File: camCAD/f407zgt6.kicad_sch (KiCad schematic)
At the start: 2 parts, among them J2 SWD Header, U3 STM32F407ZGTx

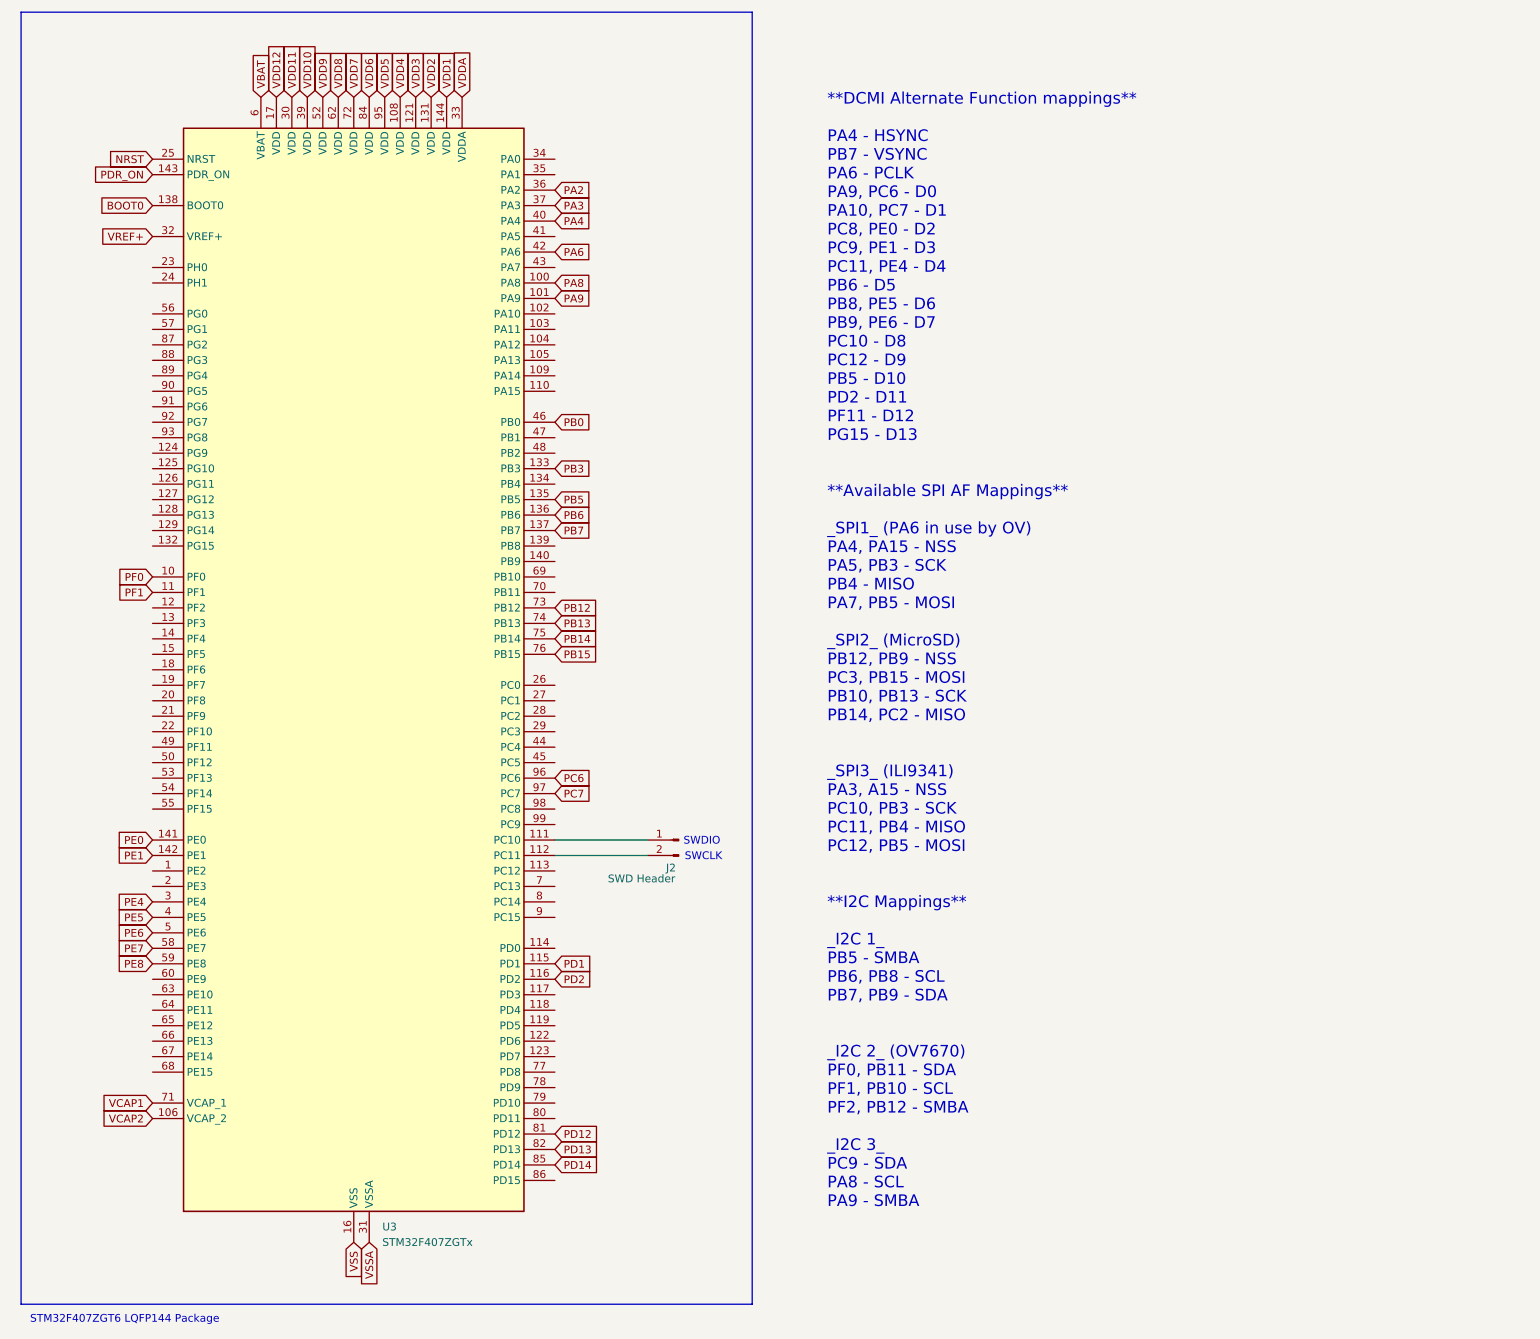
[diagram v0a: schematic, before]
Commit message: miscellaneous changes
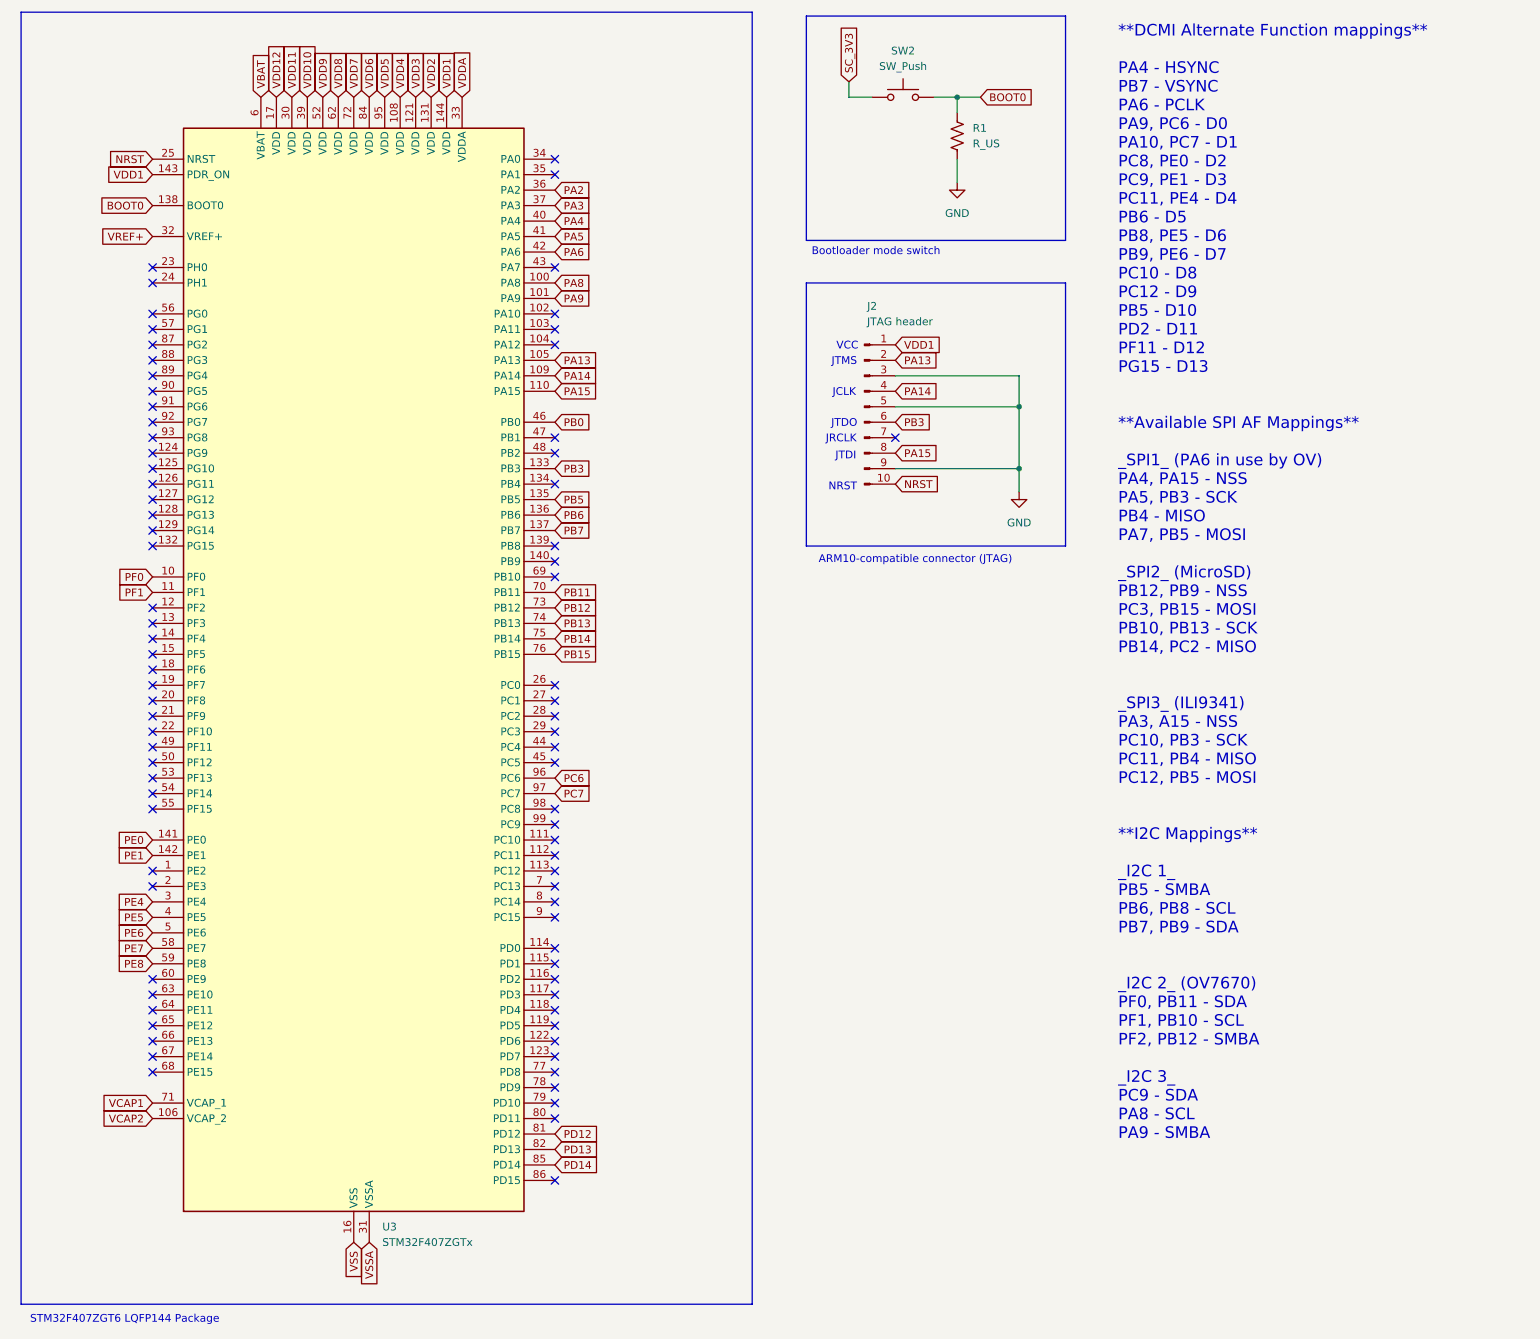
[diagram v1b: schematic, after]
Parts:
- removed J2: SWD Header, symbol Connector:Conn_01x02_Pin
- added J2: JTAG header, symbol Connector:Conn_01x10_Pin
- added R1: R_US, symbol Device:R_US
- added SW2: SW_Push, symbol Switch:SW_Push
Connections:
- net PDR_ON is gone; now on net VDD1: U3.143 (PDR_ON)
- net BOOT0: now also R1.1, SW2.2
- net NRST: now also J2.10 (Pin_10)
- net PB3: now also J2.6 (Pin_6)
- net VDD1: now also J2.1 (Pin_1)
- net PA13: now reaches U3.105 (PA13)
- net PA13: now also J2.2 (Pin_2)
- net PA14: now reaches U3.109 (PA14)
- net PA14: now also J2.4 (Pin_4)
- net PA15: now reaches U3.110 (PA15)
- net PA15: now also J2.8 (Pin_8)
- net PA5: now reaches U3.41 (PA5)
- net PB11: now reaches U3.70 (PB11)
- net PD1: no longer names the net of U3.115 (PD1)
- net PD2: no longer names the net of U3.116 (PD2)
- new net GND: J2.3 (Pin_3), J2.5 (Pin_5), J2.9 (Pin_9), R1.2
- new net SC_3V3: SW2.1
- no-connect marks 0 -> 81
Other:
- note added: "ARM10-compatible connector (JTAG)"
- note added: "Bootloader mode switch"
- note added: "JCLK"
- note added: "JRCLK"
- note added: "JTDI"
- note added: "JTDO"
- note added: "JTMS"
- note added: "NRST"
- note added: "VCC"
- note removed: "SWCLK"
- note removed: "SWDIO"
